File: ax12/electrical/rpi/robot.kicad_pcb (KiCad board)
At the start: 2 copper layers, 29.8 x 63.5 mm, 12 parts, among them J1 Raspberry_Pi_2_3, J2 IMU, J3 Power 5V/5A, J4 i2c, J6 Power/Data Input, J7 Audio, Q1 BSS138, U2 74LVC1G125, U3 74LVC1G126

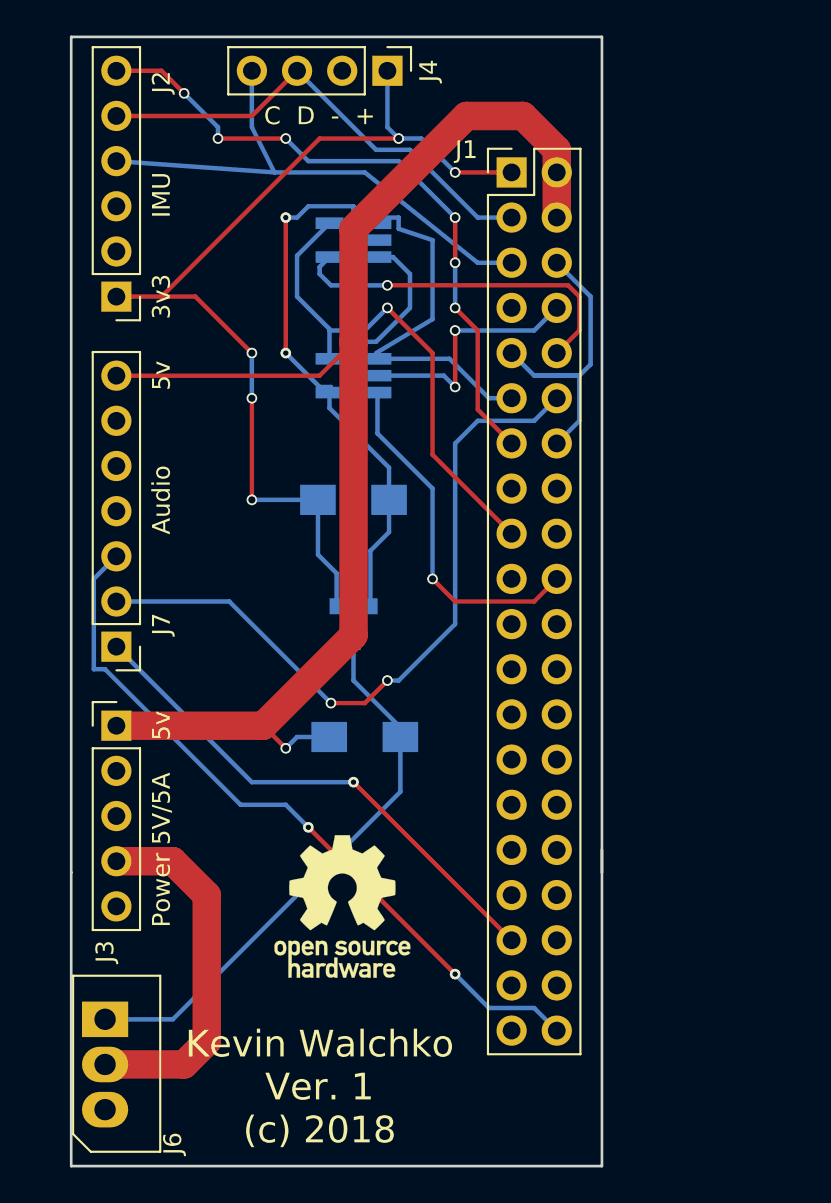
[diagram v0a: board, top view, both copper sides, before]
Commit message: up
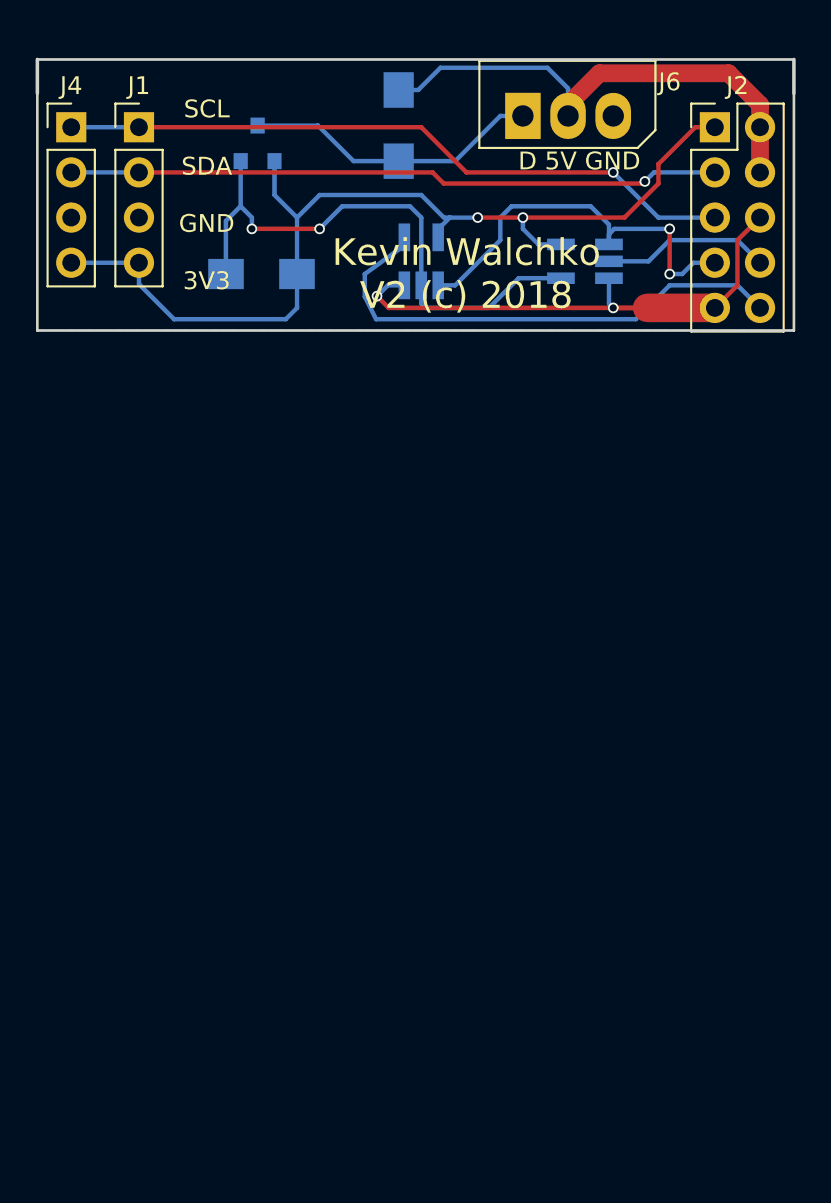
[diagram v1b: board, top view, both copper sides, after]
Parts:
- removed J3: Power 5V/5A, Pin_Headers:Pin_Header_Straight_1x05_Pitch2.54mm
- removed J7: Audio, Pin_Headers:Pin_Header_Straight_1x07_Pitch2.54mm
- removed REF***: , Symbols:OSHW-Logo_7.5x8mm_SilkScreen
- J1: value Raspberry_Pi_2_3 -> i2c; footprint Pin_Headers:Pin_Header_Straight_2x20_Pitch2.54mm -> Pin_Headers:Pin_Header_Straight_1x04_Pitch2.54mm
- J2: value IMU -> Pi Header; footprint Pin_Headers:Pin_Header_Straight_1x06_Pitch2.54mm -> Pin_Headers:Pin_Header_Straight_2x05_Pitch2.54mm
- U2: value 74LVC1G125 -> 74-125
- U3: value 74LVC1G126 -> 74-126
- moved J6 56.0 mm to (159.4, 59.1), turned to 0 degrees
- moved J2 35.0 mm to (170.2, 59.7), turned to 0 degrees
- moved R2 34.4 mm to (152.4, 59.6), turned to 270 degrees
- moved Q1 27.6 mm to (144.5, 60.6), turned to 90 degrees
- moved J1 21.1 mm to (137.8, 59.7)
- moved J4 18.1 mm to (134.0, 59.7), turned to 0 degrees
- moved U3 14.5 mm to (162.9, 67.2)
- moved R3 13.7 mm to (144.7, 67.9), turned to 180 degrees
- moved U2 3.99 mm to (153.7, 67.2), turned to 90 degrees
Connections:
- J1 pad 1: +3V3 -> SCL
- J1 pad 2: +5V -> SDA
- J1 pad 3: Net-(J1-Pad3) -> GND
- J1 pad 4: +5V -> +3V3
- J2 pad 2: (no net) -> +5V
- J2 pad 3: GND -> SDA
- J2 pad 4: Net-(J1-Pad5) -> +5V
- J2 pad 5: Net-(J1-Pad3) -> SCL
- J2 pad 6: IMU-RST -> GND
- J4 pad 1: +3V3 -> SCL
- J4 pad 2: GND -> SDA
- J4 pad 3: Net-(J1-Pad3) -> GND
- J4 pad 4: Net-(J1-Pad5) -> +3V3
- J6 pad 2: +12V -> +5V
- U2 pad 5: VCC -> +3V3
- U3 pad 5: VCC -> +3V3
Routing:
- net +5V: track 78.1 -> 28.8 mm, vias 1 -> 0
- net DIN: track 41.3 -> 0.00 mm, vias 2 -> 0
- net BCLK: track 40.2 -> 0.00 mm, vias 2 -> 0
- net SCL: track 0.00 -> 38.3 mm, vias 0 -> 1
- net IMU-RST: track 36.9 -> 0.00 mm, vias 6 -> 0
- net SDA: track 0.00 -> 36.7 mm, vias 0 -> 1
- net Net-(J1-Pad5): track 30.0 -> 0.00 mm
- net LRC: track 29.1 -> 0.00 mm, vias 1 -> 0
- net VCC: track 28.5 -> 0.00 mm, vias 1 -> 0
- net Net-(J1-Pad3): track 26.7 -> 0.00 mm
- net +12V: track 20.4 -> 0.00 mm
- net GND: track 51.0 -> 30.9 mm, vias 1 -> 2
- net DATA: track 31.4 -> 16.8 mm
- net RXI: track 20.0 -> 28.8 mm, vias 1 -> 0
- net TXO: track 14.0 -> 9.51 mm, vias 2 -> 0
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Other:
- board size 29.8 x 63.5 mm -> 42.5 x 15.2 mm
- board text added: "D 5V GND"
- board text added: "Kevin Walchko V2 (c) 2018"
- board text added: "SCL SDA GND 3V3"
- board text removed: "3v3"
- board text removed: "5v"
- board text removed: "C D - +"
- board text removed: "Kevin Walchko Ver. 1 (c) 2018"
